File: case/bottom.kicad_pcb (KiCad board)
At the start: 2 copper layers, 135 x 95.7 mm, 6 parts

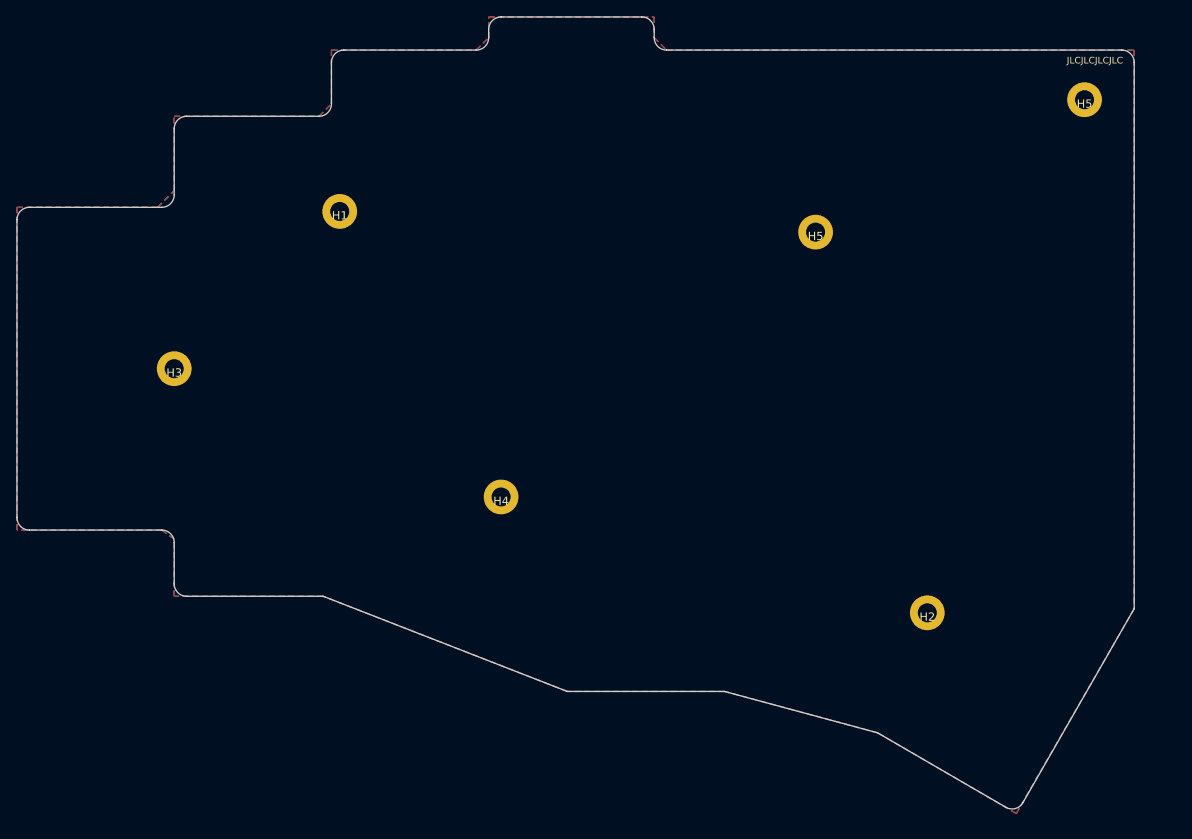
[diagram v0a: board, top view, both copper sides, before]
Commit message: update case files
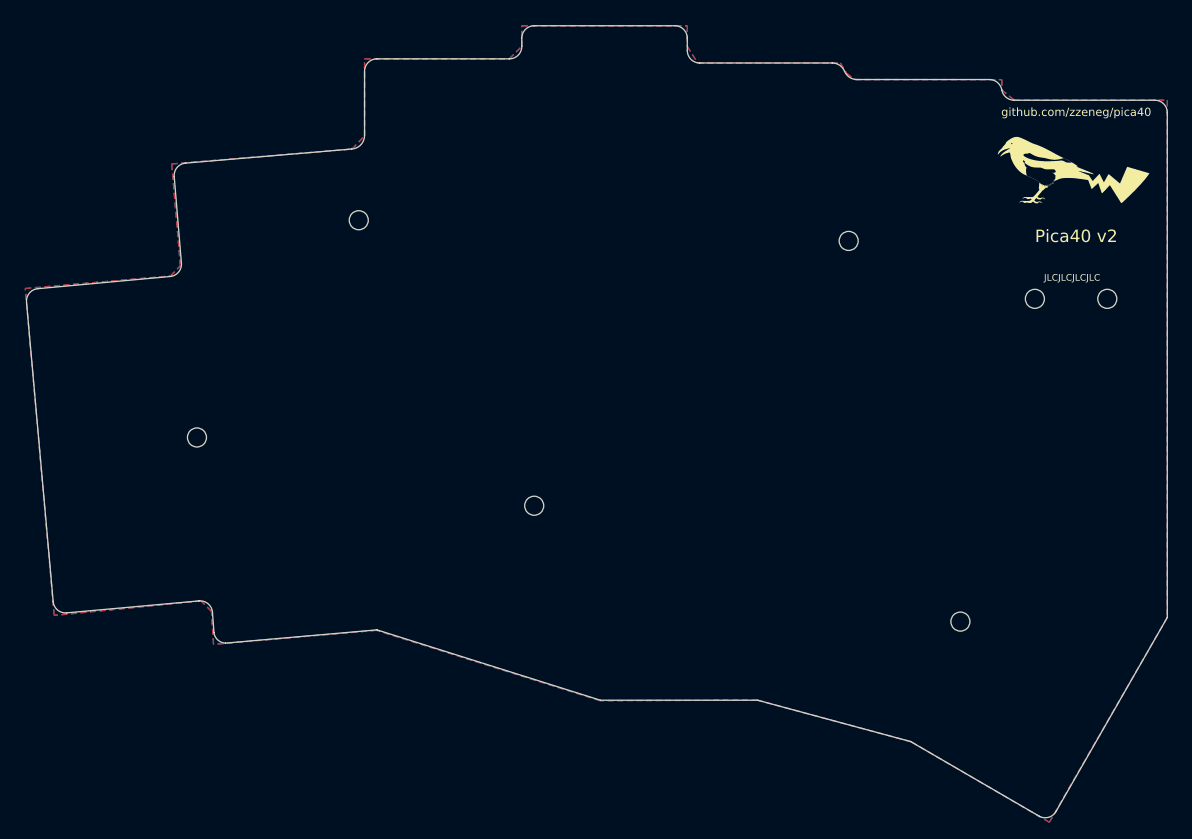
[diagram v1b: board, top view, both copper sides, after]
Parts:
- removed the H5 at (198.0, 60.0)
- removed the H5 at (165.5, 76.0)
- added G***: LOGO, pica:logo, F.Cu at (195.5, 68.5)
- added G***: LOGO, pica:logo, B.Cu at (198.0, 69.0)
- added H5: MountingHole, kbd:thread_m2, F.Cu at (169.5, 77.1)
- added H6: MountingHole, kbd:thread_m2, F.Cu at (192.0, 84.1)
- added H7: MountingHole, kbd:thread_m2, F.Cu at (200.8, 84.1)
- H1, H2, H3, H4: footprint kbd:M2_Hole_TH -> kbd:thread_m2
- moved H3 8.75 mm to (90.8, 100.8), turned to 5 degrees
- moved H2 4.14 mm to (183.0, 123.1)
- moved H4 4.14 mm to (131.5, 109.1)
- moved H1 2.53 mm to (110.3, 74.6)
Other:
- board size 135 x 95.7 mm -> 137.8 x 95.7 mm
- board text added: "Pica40 v2"
- board text added: "github.com/zzeneg/pica40"
